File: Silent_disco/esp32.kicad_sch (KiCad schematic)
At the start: 8 parts, among them SW1 SW_Push, SW2 SW_Push, U5 ESP32-WROOM-32E

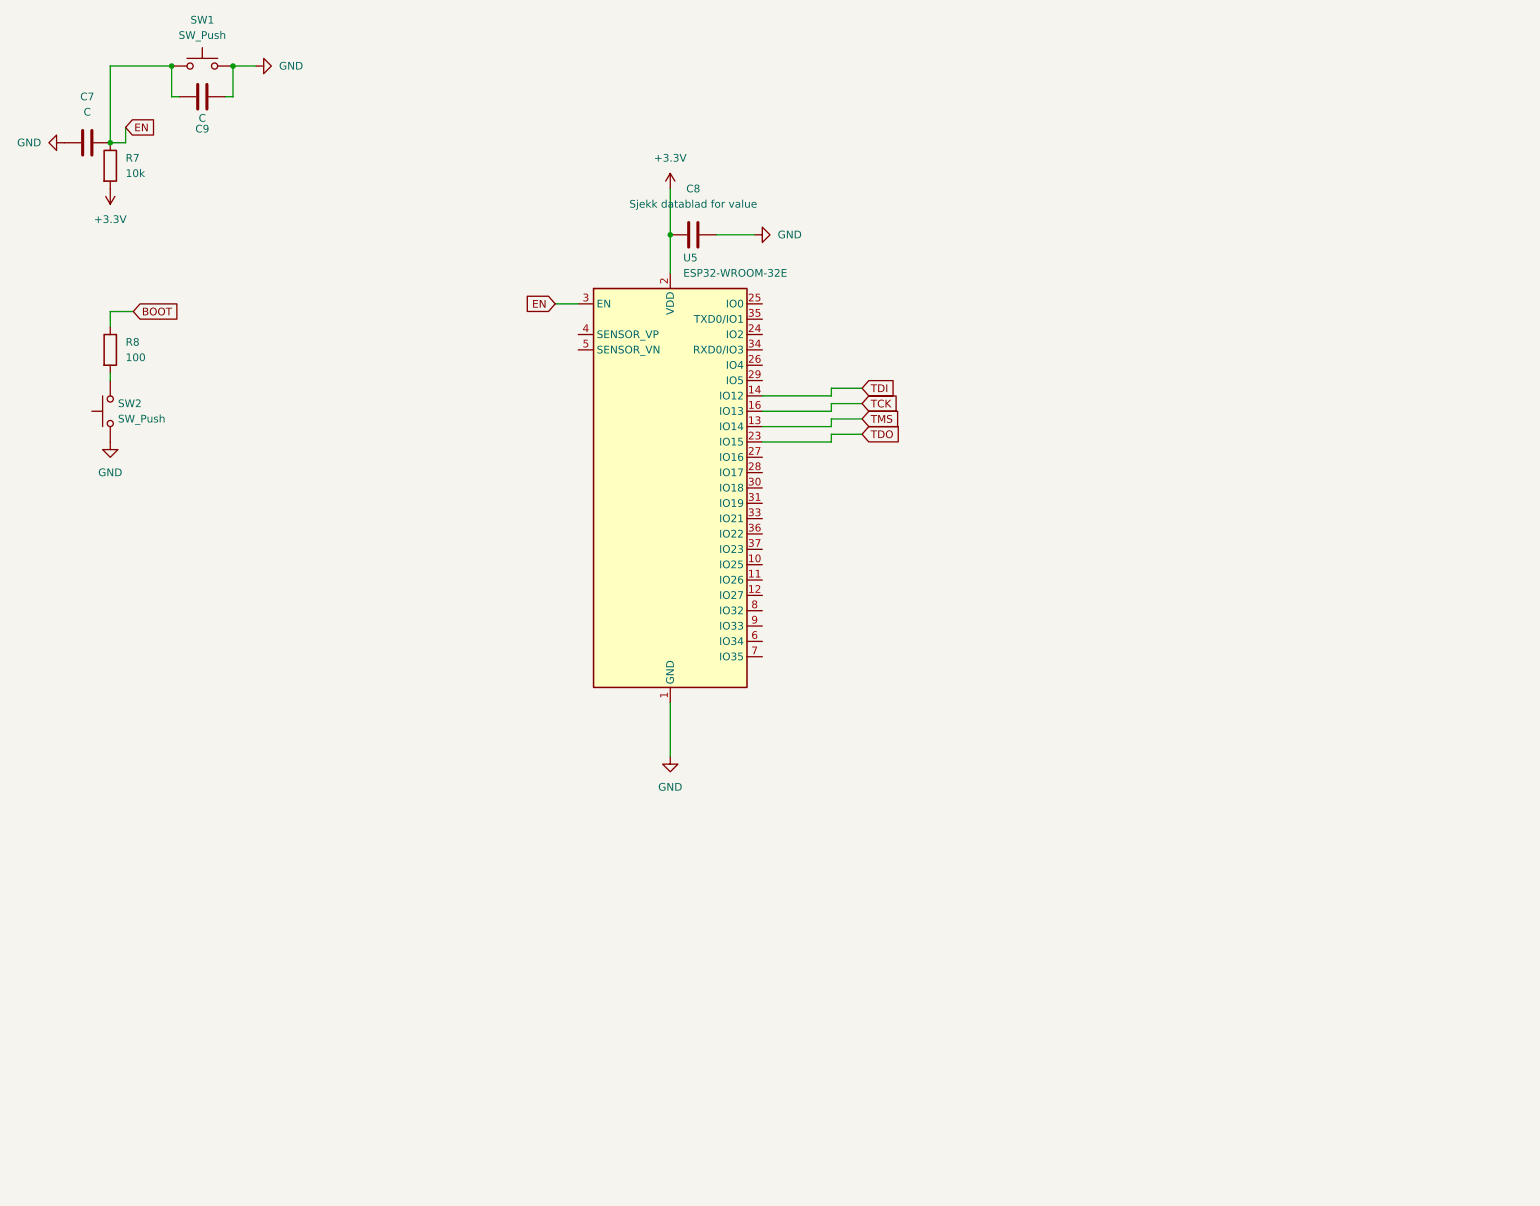
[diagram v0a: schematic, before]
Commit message: Change ic charging ic
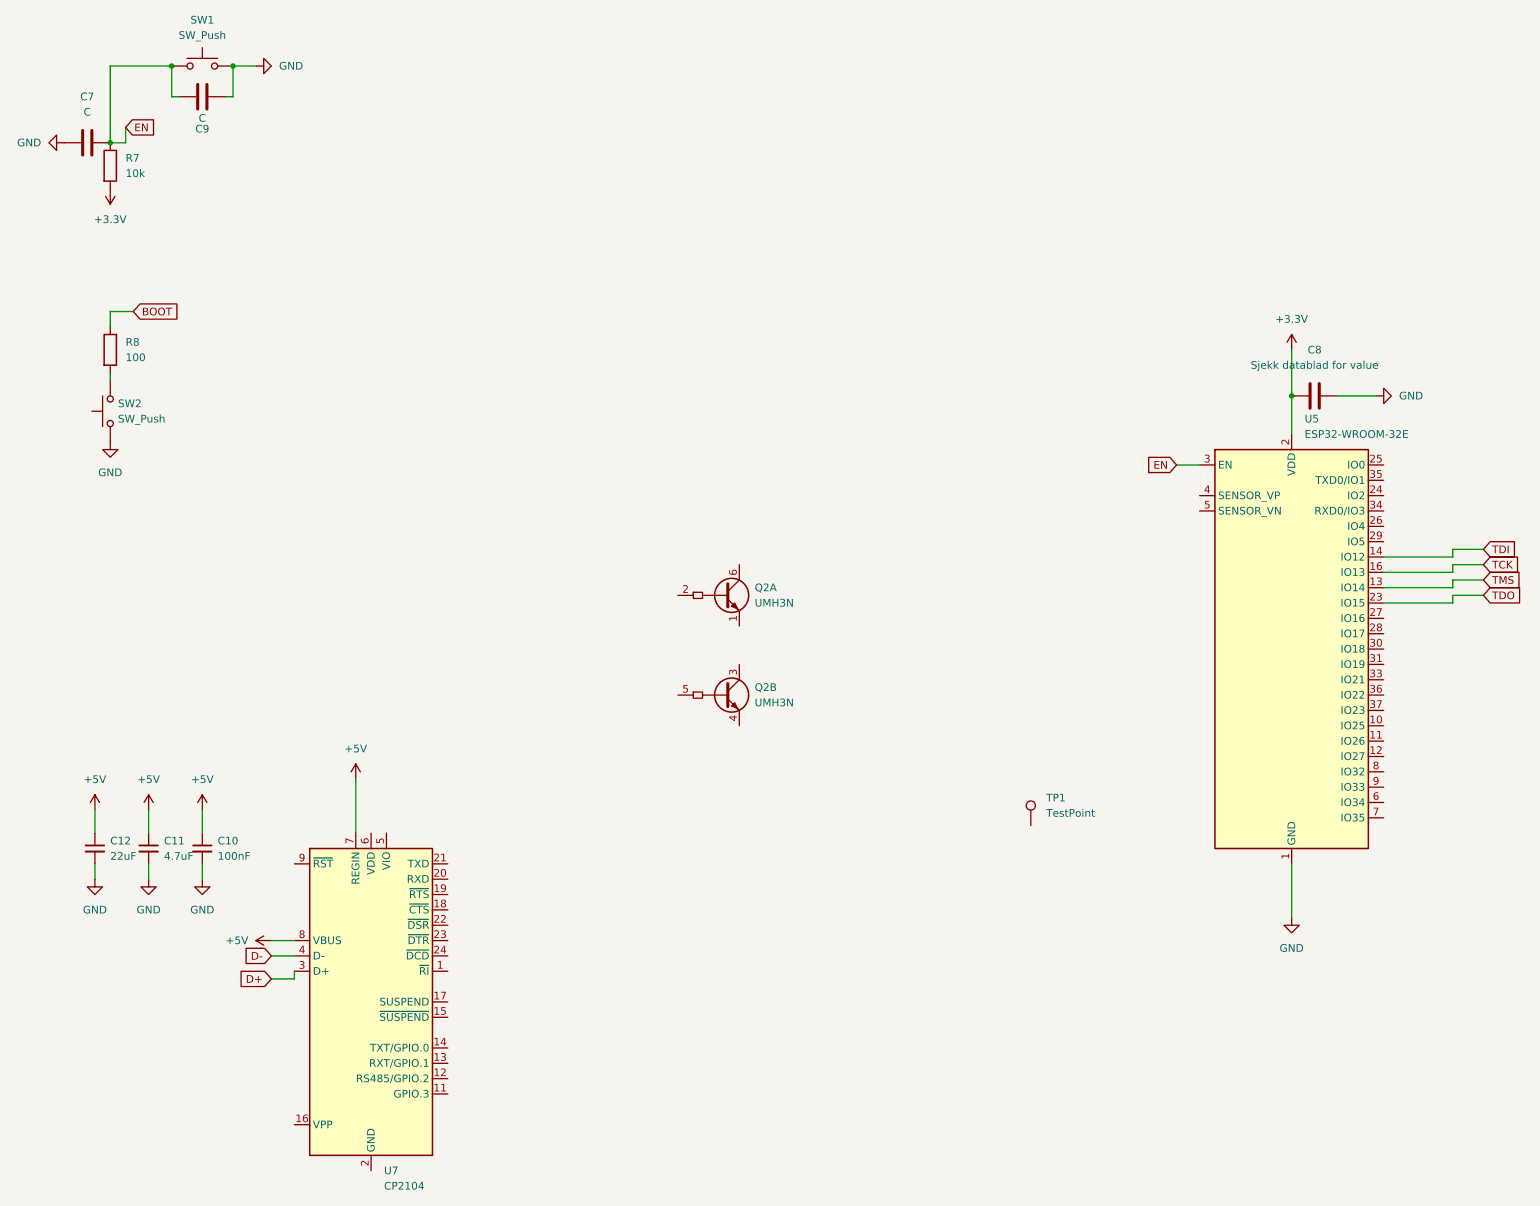
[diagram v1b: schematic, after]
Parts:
- added C10: 100nF, symbol Device:C_Small
- added C11: 4.7uF, symbol Device:C_Small
- added C12: 22uF, symbol Device:C_Small
- added Q2: UMH3N, Package_TO_SOT_SMD:SOT-363_SC-70-6, symbol Transistor_BJT:UMH3N
- added TP1: TestPoint, symbol Connector:TestPoint
- added U7: CP2104, Package_DFN_QFN:QFN-24-1EP_4x4mm_P0.5mm_EP2.6x2.6mm, symbol Interface_USB:CP2104
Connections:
- net GND: now also C10.2, C11.2, C12.2
- new net: U7.2 (GND), U7.25 (GND)
- new net +5V: C10.1, C11.1, C12.1, U7.7 (REGIN), U7.8 (VBUS)
- new net D+: U7.3 (D+)
- new net D-: U7.4 (D-)
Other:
- moved on the sheet: C8, U5
